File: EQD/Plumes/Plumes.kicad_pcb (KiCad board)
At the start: 2 copper layers, 61 x 52.9 mm, 44 parts, among them J1 Conn_01x05_Pin, SW1 On-Off-On, U1 TL074, U2 LTC1044

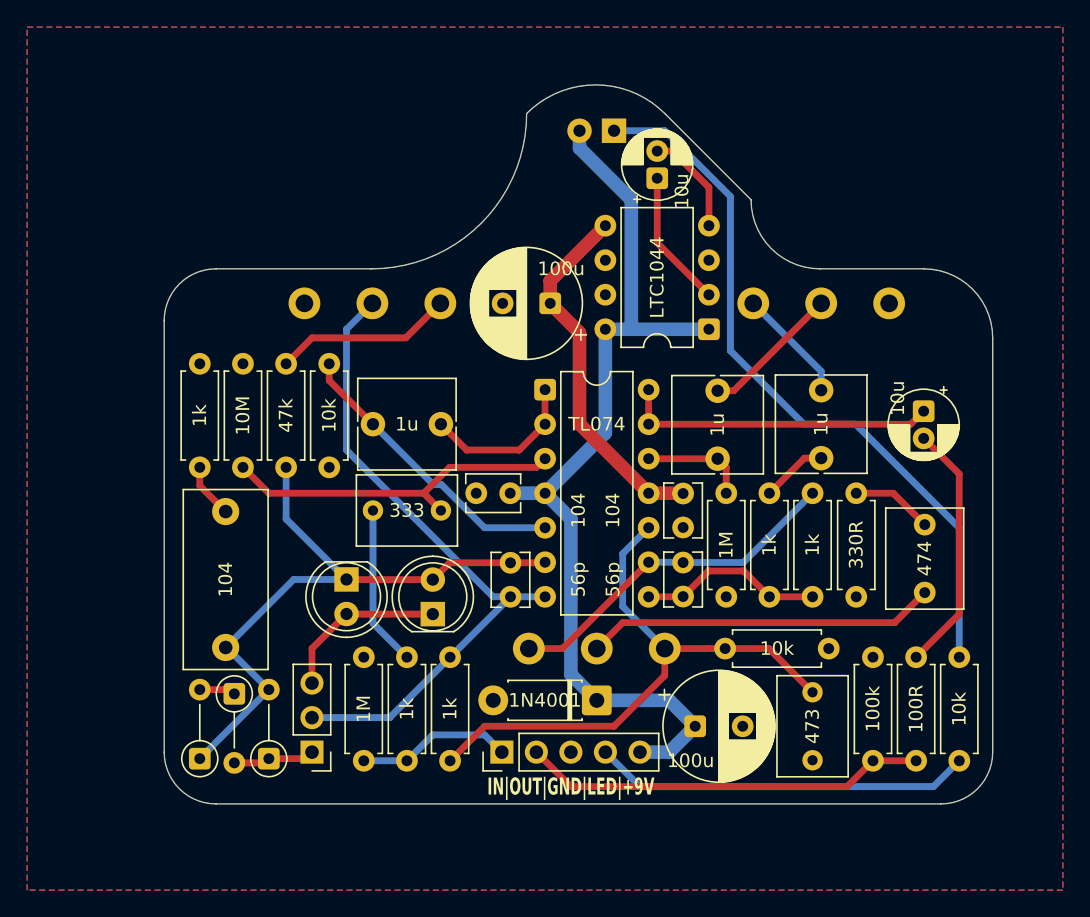
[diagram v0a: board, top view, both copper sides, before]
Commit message: feat: コネクタピンを追加
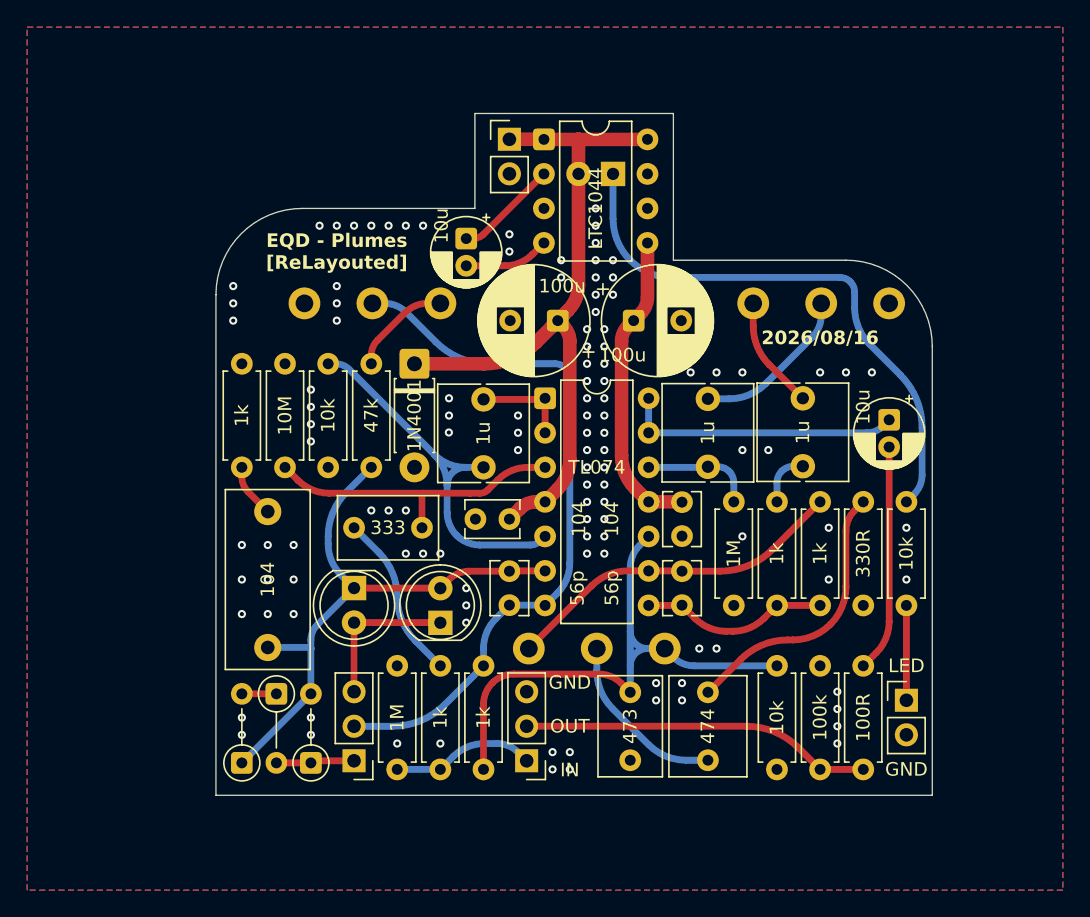
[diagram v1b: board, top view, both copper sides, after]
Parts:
- added J2: Power, Connector_PinHeader_2.54mm:PinHeader_1x02_P2.54mm_Vertical, F.Cu at (99.1, 33.6)
- added J3: LED, Connector_PinHeader_2.54mm:PinHeader_1x02_P2.54mm_Vertical, F.Cu at (128.3, 74.9)
- C1, C6: footprint Capacitor_THT:C_Rect_L7.2mm_W5.0mm_P5.00mm -> Capacitor_THT:C_Rect_L7.2mm_W4.5mm_P5.00mm_FKS2_FKP2_MKS2_MKP2
- J1: value Conn_01x05_Pin -> I/O; footprint Connector_PinHeader_2.54mm:PinHeader_1x05_P2.54mm_Vertical -> Connector_PinHeader_2.54mm:PinHeader_1x03_P2.54mm_Vertical
- moved C10 31.5 mm to (102.6, 47.0), turned to 180 degrees
- moved D7 28.2 mm to (92.1, 50.2), turned to -90 degrees
- moved C5 20.2 mm to (113.7, 79.3)
- moved U2 18.5 mm to (101.6, 33.7), turned to 0 degrees
- moved C12 14.7 mm to (95.9, 41.0), turned to -90 degrees
- moved C6 13.4 mm to (108.0, 79.3)
- moved R12 12.1 mm to (128.3, 67.9)
- moved R8 9.67 mm to (118.7, 80.0), turned to 90 degrees
- moved R6 6.27 mm to (88.9, 57.8)
- moved C14 6.27 mm to (108.2, 47.0), turned to 0 degrees
- moved R14 3.94 mm to (125.1, 72.4)
- moved R15 3.94 mm to (121.9, 72.4)
- moved C2 3.63 mm to (97.2, 52.8), turned to -90 degrees
- moved D6 3.18 mm to (106.7, 36.2)
- moved SW1 3.16 mm to (87.6, 79.4)
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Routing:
- net /LED: track 27.9 -> 6.98 mm
- net +9V: track 70.0 -> 54.3 mm
- net Net-(C5-Pad2): track 6.00 -> 20.4 mm
- net Net-(C5-Pad1): track 25.8 -> 13.1 mm
- net Net-(D6-K): track 53.7 -> 41.5 mm
- net Net-(U1B-+): track 21.6 -> 29.7 mm
- net Net-(R6-Pad2): track 13.2 -> 7.48 mm
- net Net-(U1A--): track 11.8 -> 7.04 mm
- net -9V: track 26.9 -> 22.8 mm
- net /OUTPUT: track 29.8 -> 25.8 mm
- net Net-(SW1-B): track 49.0 -> 52.8 mm
- net Net-(D1-K): track 47.9 -> 44.6 mm
- net Net-(U1A-+): track 25.9 -> 23.0 mm
- net Net-(U1D--): track 23.2 -> 20.6 mm
- net Net-(U2-CAP+): track 10.1 -> 7.63 mm
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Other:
- board size 61 x 52.9 mm -> 52.7 x 50.2 mm
- board text added: "+9V"
- board text added: "2026/08/16"
- board text added: "EQD - Plumes [ReLayouted]"
- board text added: "GND"
- board text added: "GND OUT IN"
- board text added: "LED"
- board text removed: "EQD - Plumes [ReLayouted] 2026/08/16"
- board text removed: "IN|OUT|GND|LED|+9V"
